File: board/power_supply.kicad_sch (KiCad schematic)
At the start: 21 parts

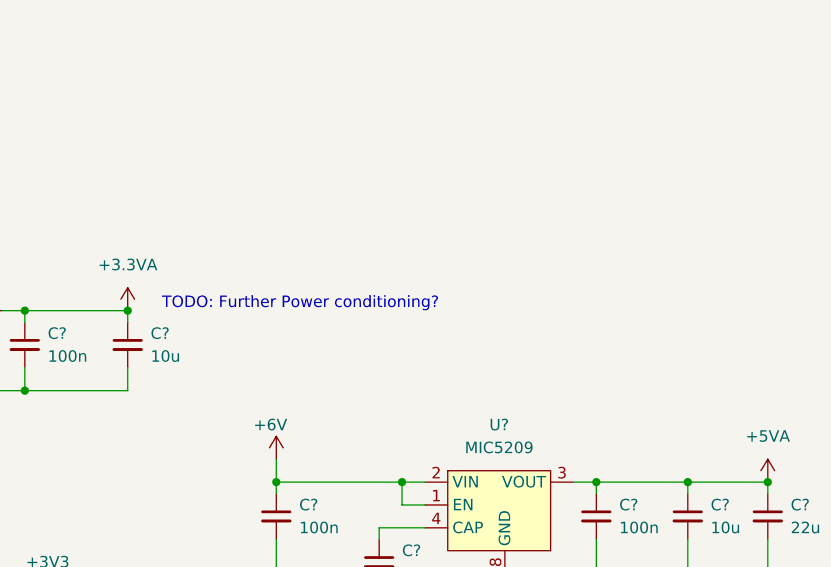
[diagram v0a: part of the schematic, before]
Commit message: updated schematic after review
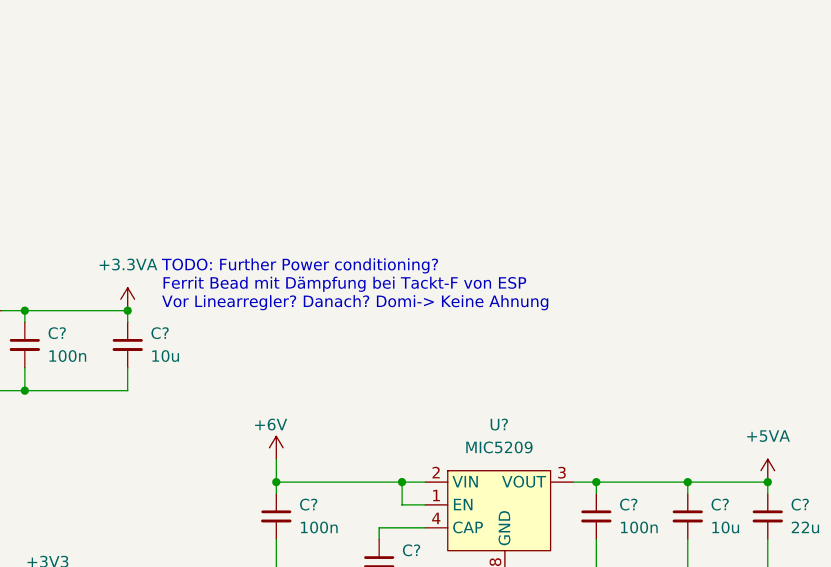
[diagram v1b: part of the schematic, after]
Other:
- note added: "TODO: Further Power conditioning? Ferrit Bead mit Dämpfung bei Tackt-F von ESP Vor Linearregler? Danach? Domi-> Keine Ahnung"
- note removed: "TODO: Further Power conditioning?"
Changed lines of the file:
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@@
     (stroke (width 0) (type default) (color 0 0 0 0))
   )
-  (text "TODO: Further Power conditioning?" (at 170.18 101.6 0)
+  (text "TODO: Further Power conditioning?\nFerrit Bead mit Dämpfung bei Tackt-F von ESP\nVor Linearregler? Danach? Domi-> Keine Ahnung"
+    (at 170.18 101.6 0)
     (effects (font (size 1.27 1.27)) (justify left bottom))
   )

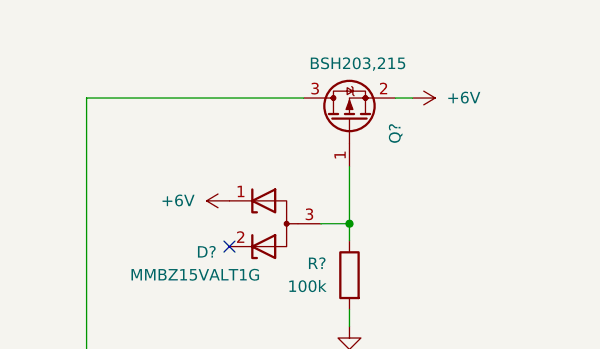
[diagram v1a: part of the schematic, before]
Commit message: updated schematic
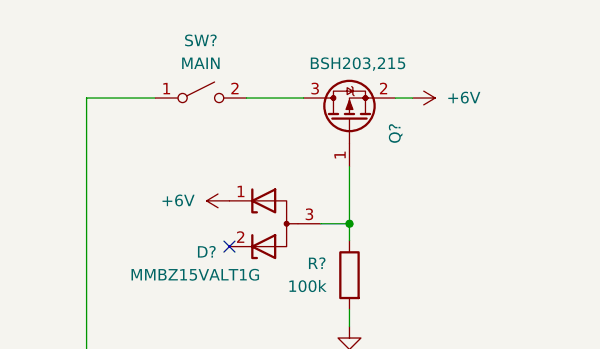
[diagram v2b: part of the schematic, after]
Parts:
- added SW?: MAIN, symbol Switch:SW_SPST
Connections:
- net at BT?.1 (+): now also SW?.1 (A); no longer Q?.3 (D)
- new net: Q?.3 (D), SW?.2 (B)
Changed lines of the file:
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@@
+    (stroke (width 0) (type default) (color 0 0 0 0))
+  )
+  (wire (pts (xy 24.13 22.86) (xy 31.75 22.86))
     (stroke (width 0) (type default) (color 0 0 0 0))
   )
@@
     (stroke (width 0) (type default) (color 0 0 0 0))
   )
-  (wire (pts (xy 24.13 22.86) (xy 48.26 22.86))
-    (stroke (width 0) (type default) (color 0 0 0 0))
-  )
   (wire (pts (xy 24.13 60.96) (xy 24.13 62.23))
     (stroke (width 0) (type default) (color 0 0 0 0))
@@
   )
   (wire (pts (xy 237.49 120.65) (xy 237.49 121.92))
+    (stroke (width 0) (type default) (color 0 0 0 0))
+  )
+  (wire (pts (xy 41.91 22.86) (xy 48.26 22.86))
     (stroke (width 0) (type default) (color 0 0 0 0))
   )
@@
     (pin "1")
   )
+  (symbol (lib_id "Switch:SW_SPST") (at 36.83 22.86 0) (unit 1)
+    (in_bom yes) (on_board yes) (fields_autoplaced)
+    (property "Reference" "SW?" (id 0) (at 36.83 16.51 0))
+    (property "Value" "MAIN" (id 1) (at 36.83 19.05 0))
+    (property "Footprint" "" (id 2) (at 36.83 22.86 0)
+      (effects (font (size 1.27 1.27)) hide)
+    )
+    (property "Datasheet" "~" (id 3) (at 36.83 22.86 0)
+      (effects (font (size 1.27 1.27)) hide)
+    )
+    (pin "1")
+    (pin "2")
+  )
   (symbol (lib_id "Device:R") (at 53.34 42.545 0) (mirror y) (unit 1)

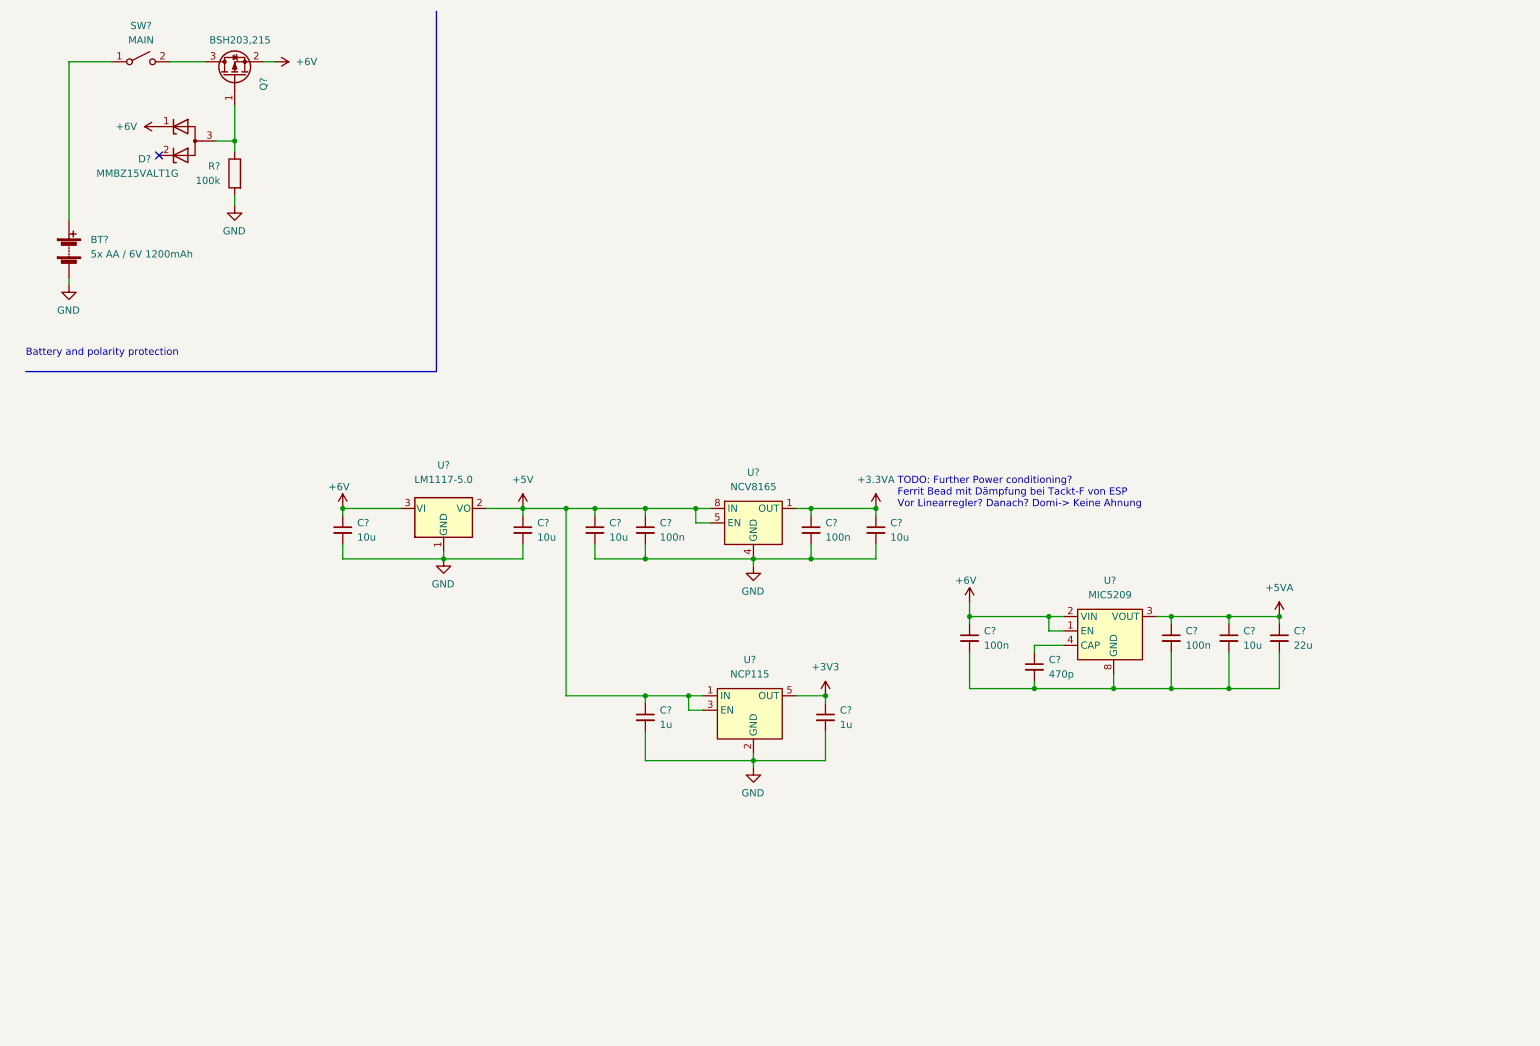
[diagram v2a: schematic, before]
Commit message: updated schematic
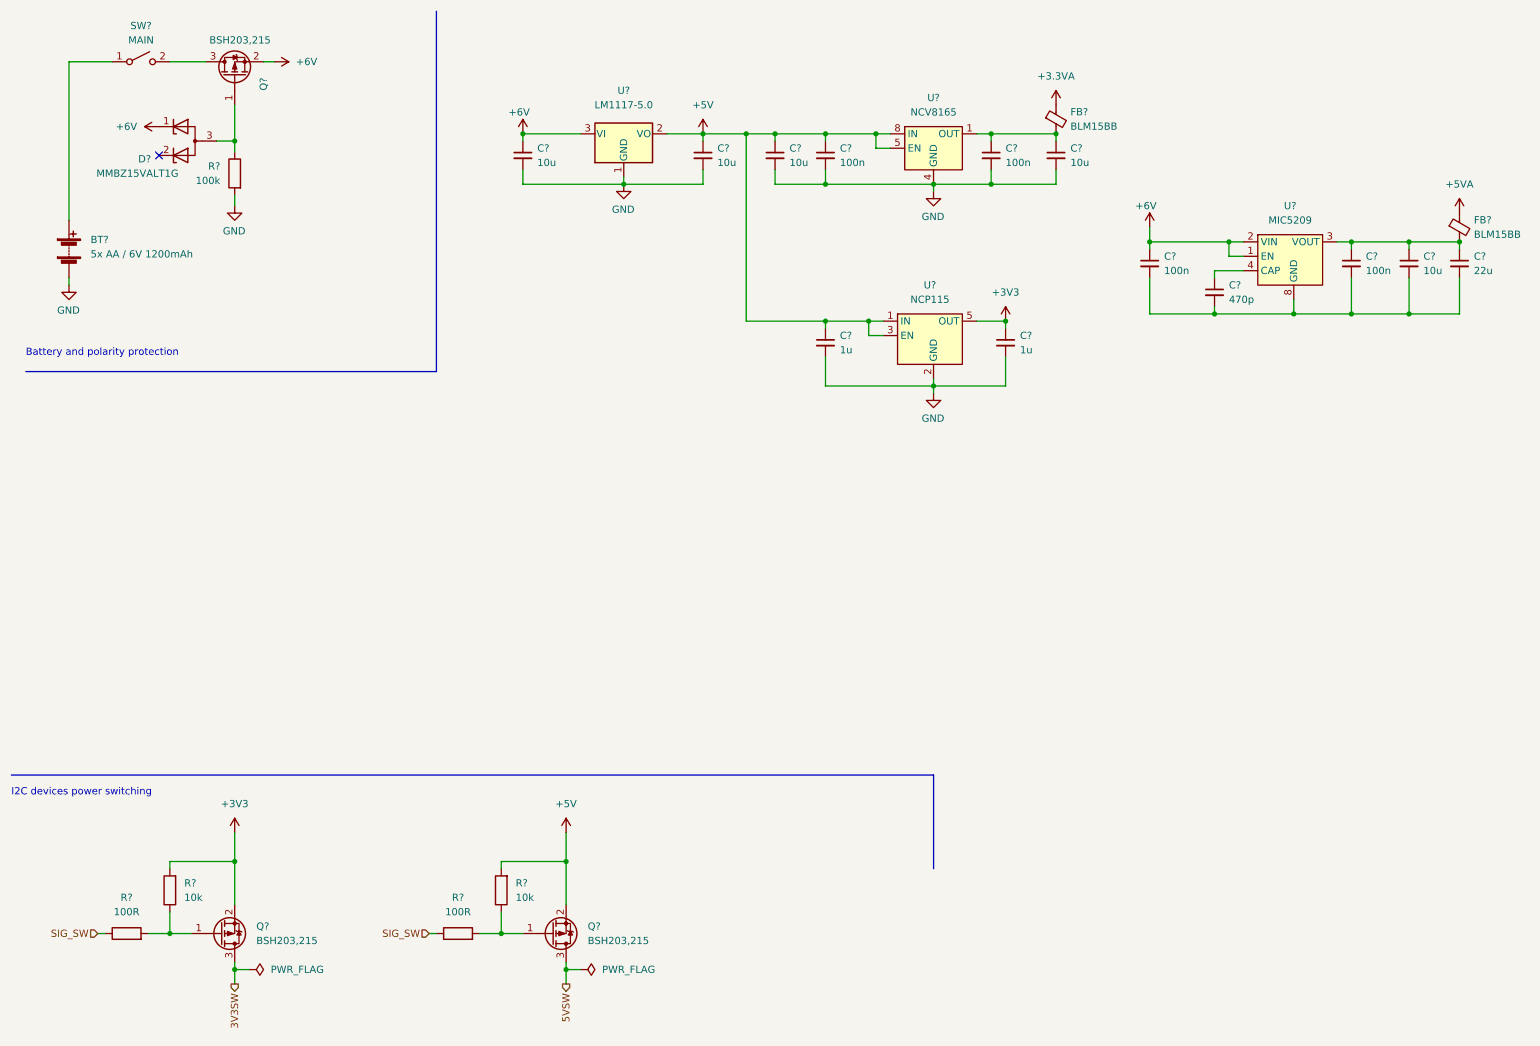
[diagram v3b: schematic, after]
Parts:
- added FB? (x2): BLM15BB, symbol Device:FerriteBead_Small
- added Q? (x2): BSH203,215, Package_TO_SOT_SMD:SOT-23, symbol Device:Q_PMOS_GSD
- added R? (x2): 10k, Resistor_SMD:R_0402_1005Metric, symbol Device:R
- added R? (x2): 100R, Resistor_SMD:R_0402_1005Metric, symbol Device:R
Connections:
- net +3.3VA: now also FB?.1; no longer C?.1, C?.1, U?.1 (OUT)
- net +3V3: now also Q?.2 (S), R?.2
- net +5V: now also Q?.2 (S), R?.2
- net +5VA: now also FB?.1; no longer C?.1, C?.1, C?.1, U?.3 (VOUT)
- new net: Q?.1 (G), R?.1, R?.2 (x2)
- new net: C?.1, C?.1, C?.1, FB?.2, U?.3 (VOUT)
- new net: C?.1, C?.1, FB?.2, U?.1 (OUT)
- new net 3V3SW: Q?.3 (D)
- new net 5VSW: Q?.3 (D)
- new net SIG_SW: R?.1, R?.1
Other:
- note added: "I2C devices power switching"
- note removed: "TODO: Further Power conditioning? Ferrit Bead mit Dämpfung bei Tackt-F von ESP Vor Linearregler? Danach? Domi-> Keine Ahnung"
- moved on the sheet: C?, U?
